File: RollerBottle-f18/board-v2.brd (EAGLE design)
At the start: 133.3 x 100 mm, 24 parts, among them IC1 7805T, J1 POWER_JACKPTH_BREAD, U1 328P

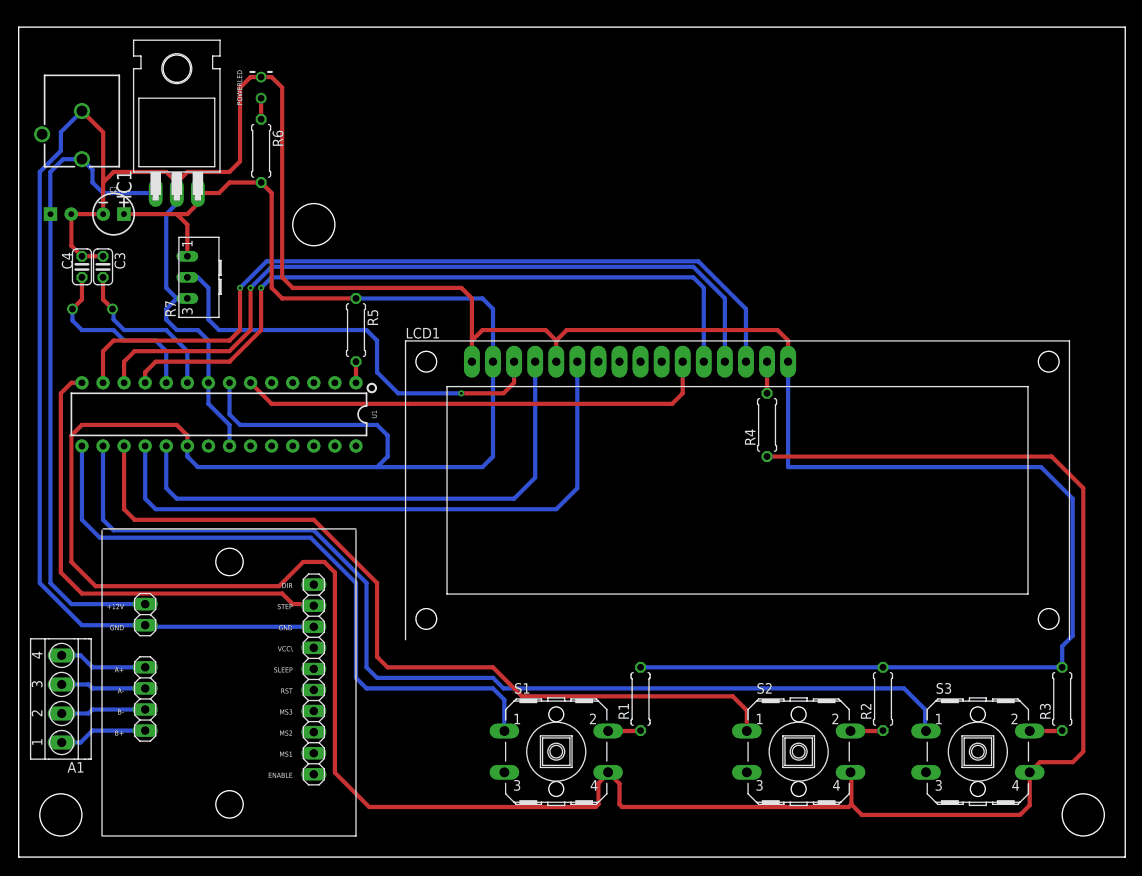
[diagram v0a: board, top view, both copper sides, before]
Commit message: Board finished
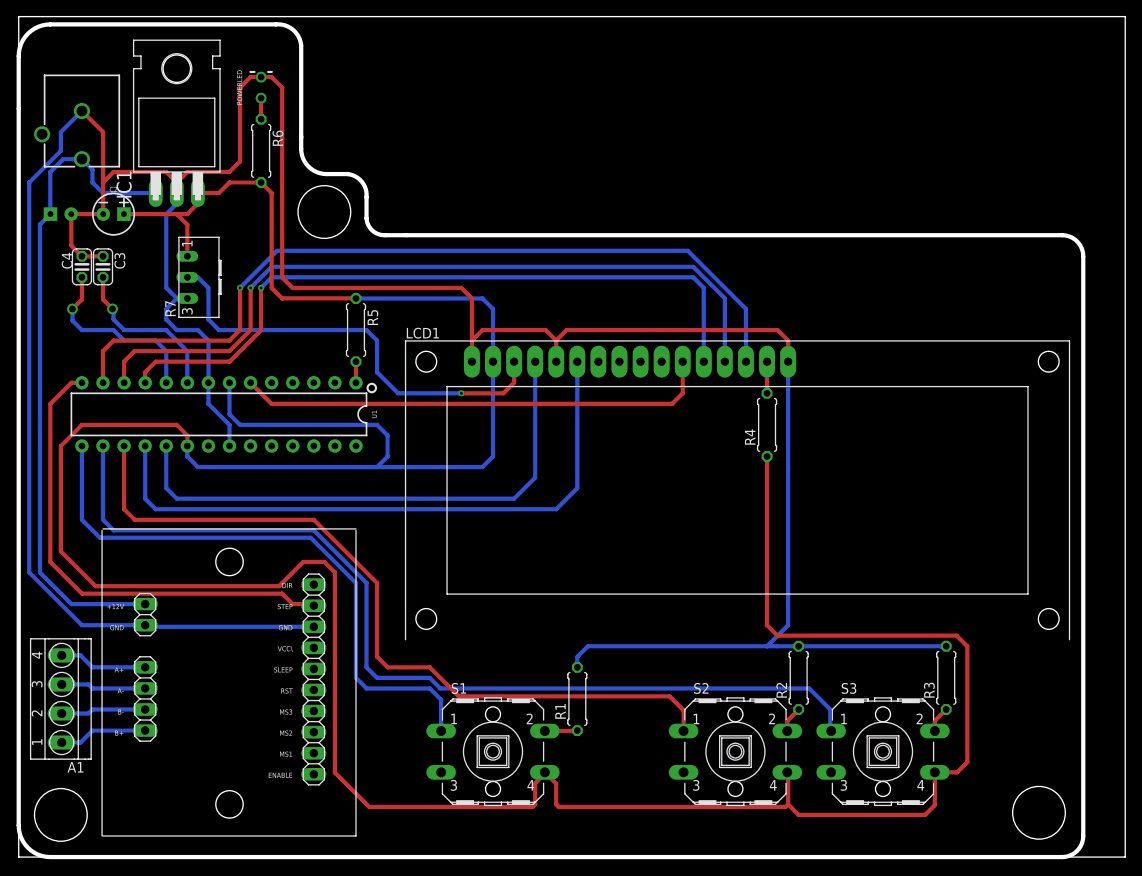
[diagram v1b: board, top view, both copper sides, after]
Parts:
- moved R3 14.2 mm to (111.8, 21.6)
- moved S3 11.4 mm to (104.1, 12.7)
- moved R2 10.5 mm to (94.0, 21.6)
- moved R1 7.62 mm to (67.3, 19.1)
- moved S2 7.62 mm to (86.4, 12.7)
- moved S1 7.62 mm to (57.1, 12.7)
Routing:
- net GND: track 412.4 -> 374.8 mm
- net +5V: track 420.7 -> 395.3 mm
- net MINUS: track 126.0 -> 114.6 mm
- net PLUS: track 100.4 -> 92.8 mm
- net MODE: track 79.2 -> 71.6 mm
- net DB7: track 97.5 -> 98.5 mm
- net +12V: track 77.9 -> 79.0 mm
- net M_STEP: track 56.8 -> 57.8 mm
- net N$15: track 3.93 -> 3.16 mm
- net N$16: track 3.93 -> 3.16 mm
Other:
- board size 133.3 x 100 mm -> 133.3 x 101.3 mm
